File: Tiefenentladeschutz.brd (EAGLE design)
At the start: 52 x 52 mm, 22 parts, among them IC1 ICL7665CSA, Q4 NMOSFET-D2PAK-7, T1 BC856B

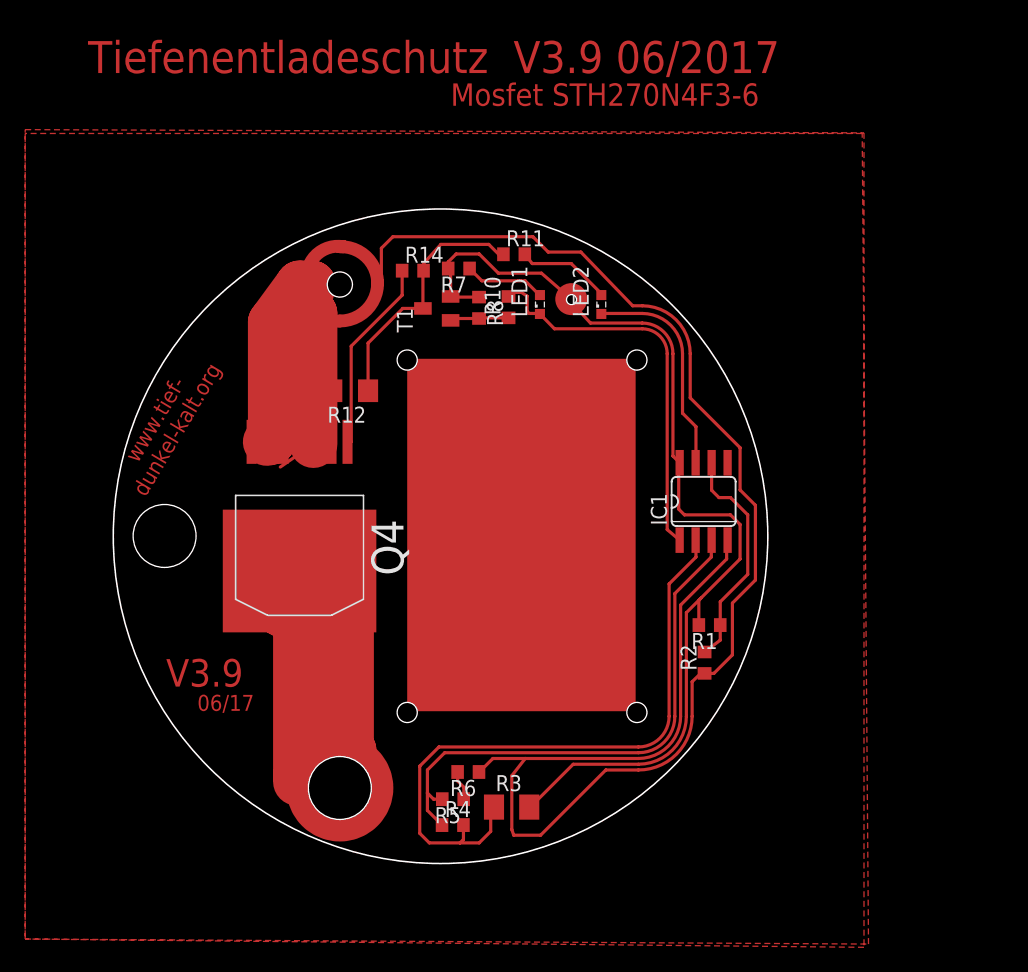
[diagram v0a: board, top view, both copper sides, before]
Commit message: Breitere Leiterbahnen und Gehäuse Modell
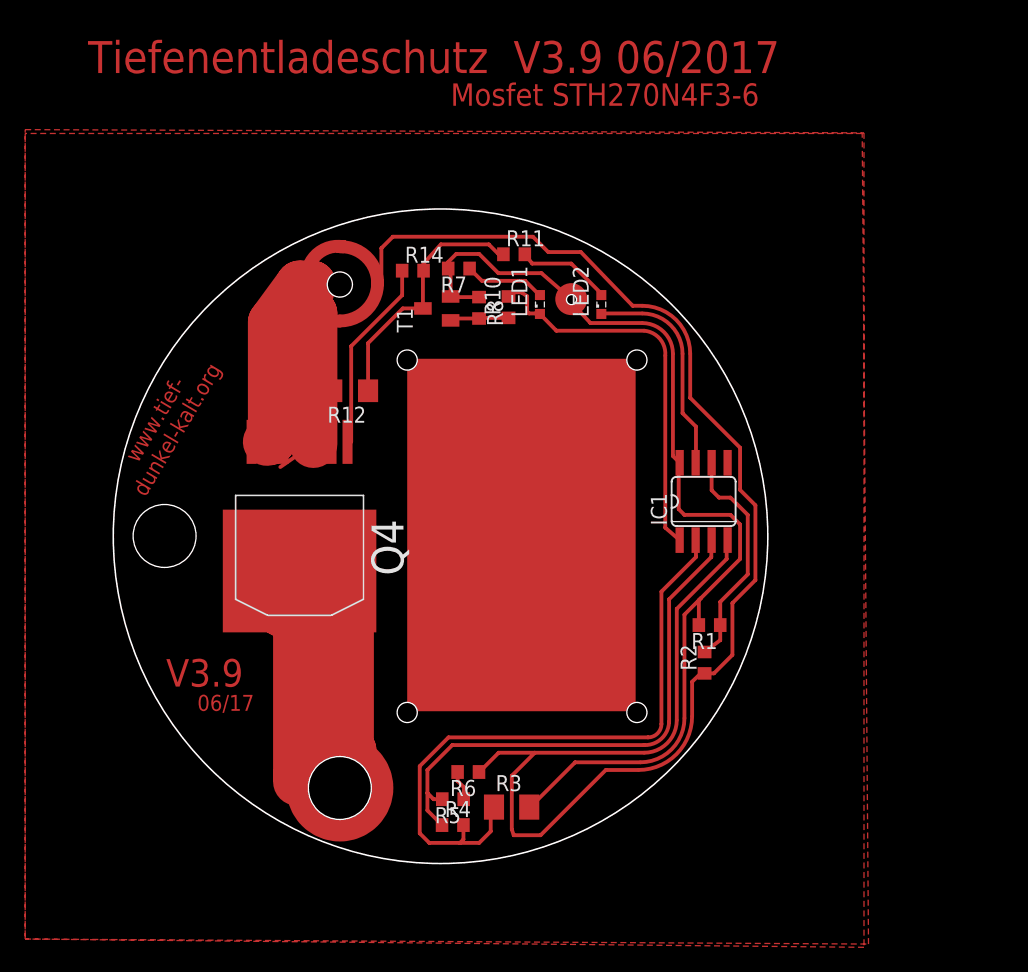
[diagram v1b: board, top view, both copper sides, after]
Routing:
- net GND: track 195.0 -> 195.9 mm
